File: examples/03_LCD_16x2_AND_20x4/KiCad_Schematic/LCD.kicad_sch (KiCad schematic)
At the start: 12 parts, among them J1 KIT DIY 5~7W QN8066, U1 LCD 16x02 or 20x04

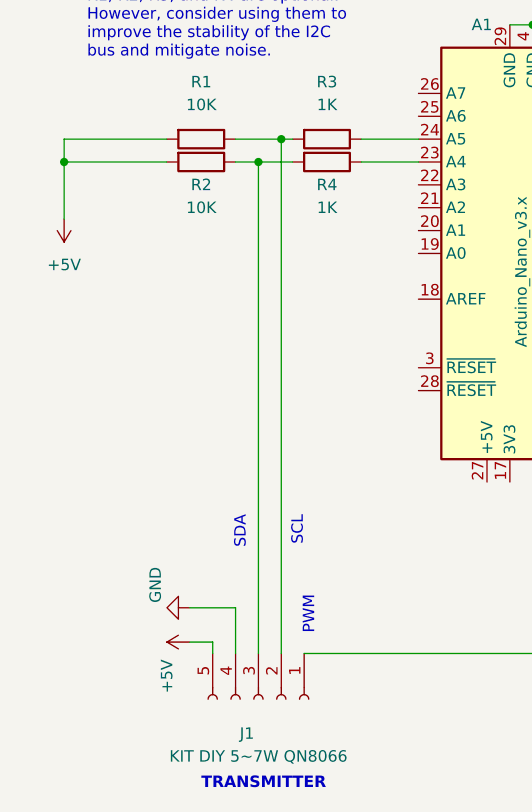
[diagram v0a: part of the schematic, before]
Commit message: DOc
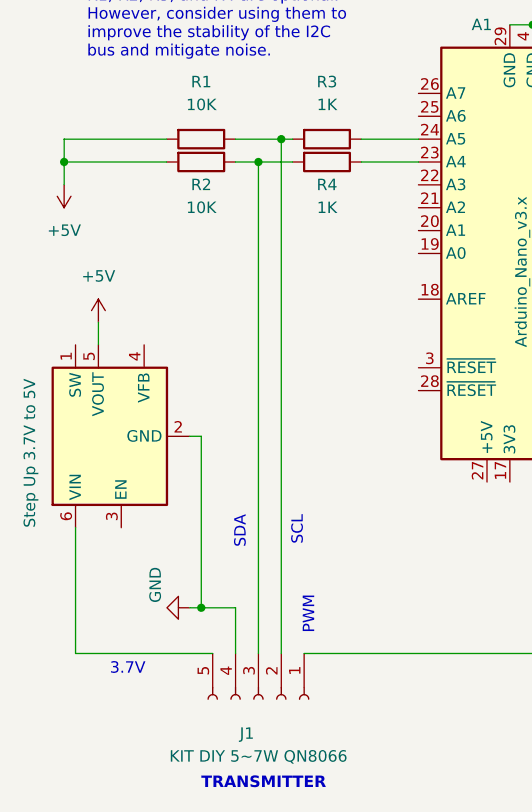
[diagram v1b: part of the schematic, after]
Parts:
- added U2: Step Up 3.7V to 5V, Package_TO_SOT_SMD:SOT-23-6, symbol Regulator_Switching:MCP1640CCH
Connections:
- net +5V: now also U2.5 (VOUT); no longer J1.5 (Pin_5)
- net GND: now also U2.2 (GND)
- new net: J1.5 (Pin_5), U2.6 (VIN)
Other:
- note added: "3.7V"
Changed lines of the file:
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@@
   (junction (at 146.05 60.96) (diameter 0) (color 0 0 0 0)
   )
+  (junction (at 34.29 88.9) (diameter 0) (color 0 0 0 0)
+  )
   (junction (at 19.05 39.37) (diameter 0) (color 0 0 0 0)
   )
@@
     (stroke (width 0) (type default))
   )
+  (wire (pts (xy 35.56 93.98) (xy 20.32 93.98))
+    (stroke (width 0) (type default))
+  )
+  (wire (pts (xy 22.86 57.15) (xy 22.86 59.69))
+    (stroke (width 0) (type default))
+  )
   (wire (pts (xy 87.63 93.98) (xy 45.72 93.98))
     (stroke (width 0) (type default))
@@
     (stroke (width 0) (type default))
   )
+  (wire (pts (xy 19.05 39.37) (xy 19.05 41.91))
+    (stroke (width 0) (type default))
+  )
   (wire (pts (xy 83.82 52.07) (xy 135.89 52.07))
     (stroke (width 0) (type default))
   )
+  (wire (pts (xy 34.29 88.9) (xy 33.02 88.9))
+    (stroke (width 0) (type default))
+  )
   (wire (pts (xy 83.82 31.75) (xy 86.36 31.75))
     (stroke (width 0) (type default))
   )
-  (wire (pts (xy 35.56 93.98) (xy 35.56 92.71))
-    (stroke (width 0) (type default))
-  )
   (wire (pts (xy 123.19 39.37) (xy 83.82 39.37))
     (stroke (width 0) (type default))
@@
     (stroke (width 0) (type default))
   )
-  (wire (pts (xy 38.1 88.9) (xy 33.02 88.9))
+  (wire (pts (xy 38.1 88.9) (xy 34.29 88.9))
     (stroke (width 0) (type default))
   )
@@
     (stroke (width 0) (type default))
   )
+  (wire (pts (xy 33.02 69.85) (xy 34.29 69.85))
+    (stroke (width 0) (type default))
+  )
   (wire (pts (xy 87.63 41.91) (xy 87.63 93.98))
     (stroke (width 0) (type default))
@@
     (stroke (width 0) (type default))
   )
+  (wire (pts (xy 20.32 93.98) (xy 20.32 80.01))
+    (stroke (width 0) (type default))
+  )
   (wire (pts (xy 156.21 24.13) (xy 166.37 24.13))
     (stroke (width 0) (type default))
   )
-  (wire (pts (xy 35.56 92.71) (xy 33.02 92.71))
+  (wire (pts (xy 34.29 69.85) (xy 34.29 88.9))
     (stroke (width 0) (type default))
   )
@@
     (stroke (width 0) (type default))
   )
+  (wire (pts (xy 43.18 36.83) (xy 43.18 93.98))
+    (stroke (width 0) (type default))
+  )
+  (wire (pts (xy 40.64 39.37) (xy 44.45 39.37))
+    (stroke (width 0) (type default))
+  )
+  (wire (pts (xy 146.05 60.96) (xy 156.21 60.96))
+    (stroke (width 0) (type default))
+  )
+  (wire (pts (xy 161.29 46.99) (xy 161.29 50.8))
+    (stroke (width 0) (type default))
+  )
   (wire (pts (xy 19.05 36.83) (xy 19.05 39.37))
-    (stroke (width 0) (type default))
-  )
-  (wire (pts (xy 43.18 36.83) (xy 43.18 93.98))
-    (stroke (width 0) (type default))
-  )
-  (wire (pts (xy 40.64 39.37) (xy 44.45 39.37))
-    (stroke (width 0) (type default))
-  )
-  (wire (pts (xy 146.05 60.96) (xy 156.21 60.96))
-    (stroke (width 0) (type default))
-  )
-  (wire (pts (xy 161.29 46.99) (xy 161.29 50.8))
-    (stroke (width 0) (type default))
-  )
-  (wire (pts (xy 19.05 39.37) (xy 19.05 45.72))
     (stroke (width 0) (type default))
   )
@@
     (effects (font (size 1.27 1.27)) (justify right bottom))
   )
+  (text "3.7V" (at 24.13 96.52 0)
+    (effects (font (size 1.27 1.27)) (justify left bottom))
+  )
   (text "R1, R2, R3, and R4 are optional.\nHowever, consider using them to \nimprove the stability of the I2C \nbus and mitigate noise."
     (at 21.59 27.94 0)
@@
         (path "/03b4fd1c-f30e-47c7-82cf-518aad4befbb"
           (reference "#PWR06") (unit 1)
+        )
+      )
+    )
+  )
+  (symbol (lib_id "Regulator_Switching:MCP1640CCH") (at 25.4 69.85 90) (unit 1)
+    (in_bom yes) (on_board yes) (dnp no)
+    (property "Reference" "U2" (at 16.51 68.58 90)
+      (effects (font (size 1.27 1.27)) (justify left) hide)
+    )
+    (property "Value" "Step Up  3.7V to 5V" (at 15.24 80.01 0)
+      (effects (font (size 1.27 1.27)) (justify left))
+    )
+    (property "Footprint" "Package_TO_SOT_SMD:SOT-23-6" (at 31.75 68.58 0)
+      (effects (font (size 1.27 1.27) italic) (justify left) hide)
+    )
+    (property "Datasheet" "http://ww1.microchip.com/downloads/en/DeviceDoc/20002234D.pdf" (at 13.97 76.2 0)
+      (effects (font (size 1.27 1.27)) hide)
+    )
+    (pin "1")
+    (pin "2")
+    (pin "3")
+    (pin "4")
+    (pin "5")
+    (pin "6")
+    (instances
+      (project "LCD"
+        (path "/03b4fd1c-f30e-47c7-82cf-518aad4befbb"
+          (reference "U2") (unit 1)
         )
       )
@@
     )
   )
-  (symbol (lib_id "power:+5V") (at 19.05 45.72 180) (unit 1)
+  (symbol (lib_id "power:+5V") (at 19.05 41.91 180) (unit 1)
     (in_bom yes) (on_board yes) (dnp no) (fields_autoplaced)
-    (property "Reference" "#PWR08" (at 19.05 41.91 0)
-      (effects (font (size 1.27 1.27)) hide)
-    )
-    (property "Value" "+5V" (at 19.05 50.8 0)
-      (effects (font (size 1.27 1.27)))
-    )
-    (property "Footprint" "" (at 19.05 45.72 0)
-      (effects (font (size 1.27 1.27)) hide)
-    )
-    (property "Datasheet" "" (at 19.05 45.72 0)
+    (property "Reference" "#PWR08" (at 19.05 38.1 0)
+      (effects (font (size 1.27 1.27)) hide)
+    )
+    (property "Value" "+5V" (at 19.05 46.99 0)
+      (effects (font (size 1.27 1.27)))
+    )
+    (property "Footprint" "" (at 19.05 41.91 0)
+      (effects (font (size 1.27 1.27)) hide)
+    )
+    (property "Datasheet" "" (at 19.05 41.91 0)
       (effects (font (size 1.27 1.27)) hide)
     )
@@
         (path "/03b4fd1c-f30e-47c7-82cf-518aad4befbb"
           (reference "#PWR08") (unit 1)
-        )
-      )
-    )
-  )
-  (symbol (lib_id "power:+5V") (at 33.02 92.71 90) (unit 1)
-    (in_bom yes) (on_board yes) (dnp no)
-    (property "Reference" "#PWR09" (at 36.83 92.71 0)
-      (effects (font (size 1.27 1.27)) hide)
-    )
-    (property "Value" "+5V" (at 30.48 96.52 0)
-      (effects (font (size 1.27 1.27)))
-    )
-    (property "Footprint" "" (at 33.02 92.71 0)
-      (effects (font (size 1.27 1.27)) hide)
-    )
-    (property "Datasheet" "" (at 33.02 92.71 0)
-      (effects (font (size 1.27 1.27)) hide)
-    )
-    (pin "1")
-    (instances
-      (project "LCD"
-        (path "/03b4fd1c-f30e-47c7-82cf-518aad4befbb"
-          (reference "#PWR09") (unit 1)
         )
       )
@@
         )
       )
+    )
+  )
+  (symbol (lib_id "power:+5V") (at 22.86 57.15 0) (unit 1)
+    (in_bom yes) (on_board yes) (dnp no) (fields_autoplaced)
+    (property "Reference" "#PWR09" (at 22.86 60.96 0)
+      (effects (font (size 1.27 1.27)) hide)
+    )
+    (property "Value" "+5V" (at 22.86 52.07 0)
+      (effects (font (size 1.27 1.27)))
+    )
+    (property "Footprint" "" (at 22.86 57.15 0)
+      (effects (font (size 1.27 1.27)) hide)
+    )
+    (property "Datasheet" "" (at 22.86 57.15 0)
+      (effects (font (size 1.27 1.27)) hide)
+    )
+    (pin "1")
+    (instances
+      (project "LCD"
+        (path "/03b4fd1c-f30e-47c7-82cf-518aad4befbb"
+          (reference "#PWR09") (unit 1)
+        )
+      )
